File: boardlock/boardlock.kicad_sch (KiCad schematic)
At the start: 0 parts

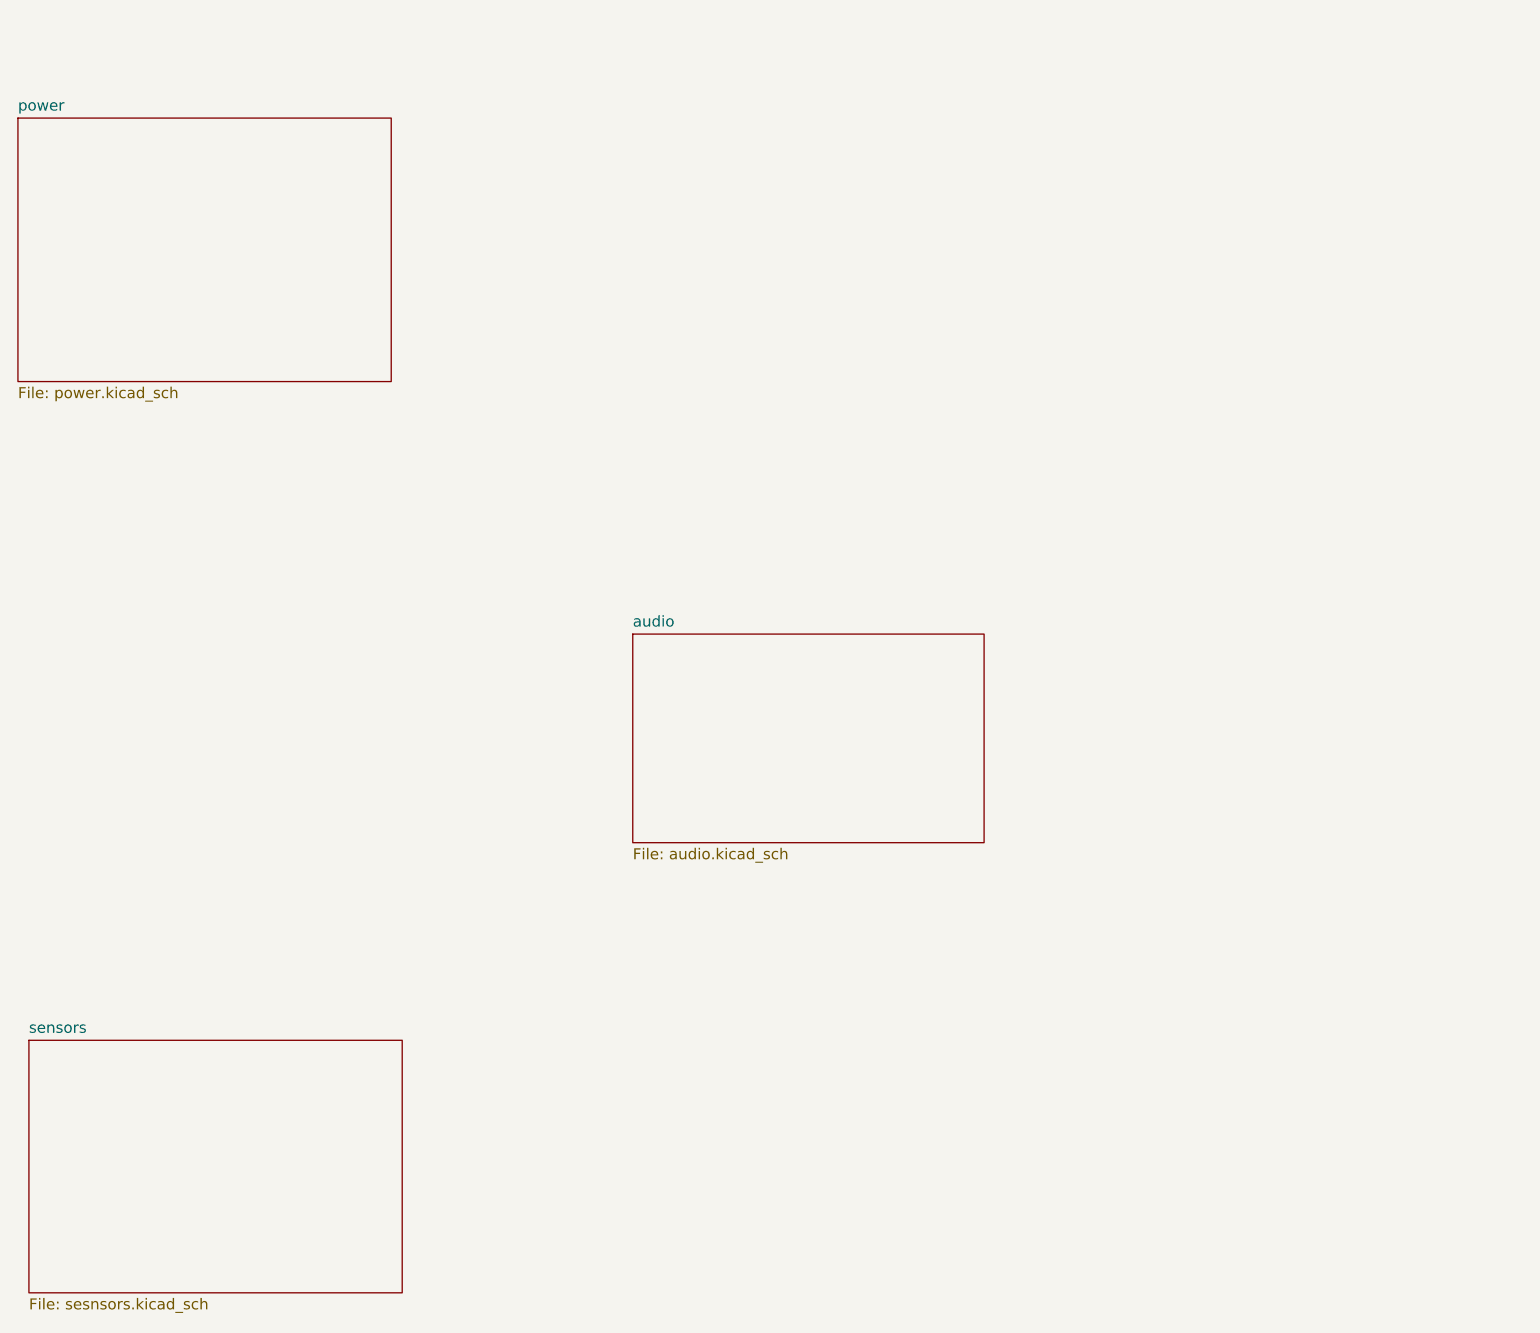
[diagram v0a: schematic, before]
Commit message: update
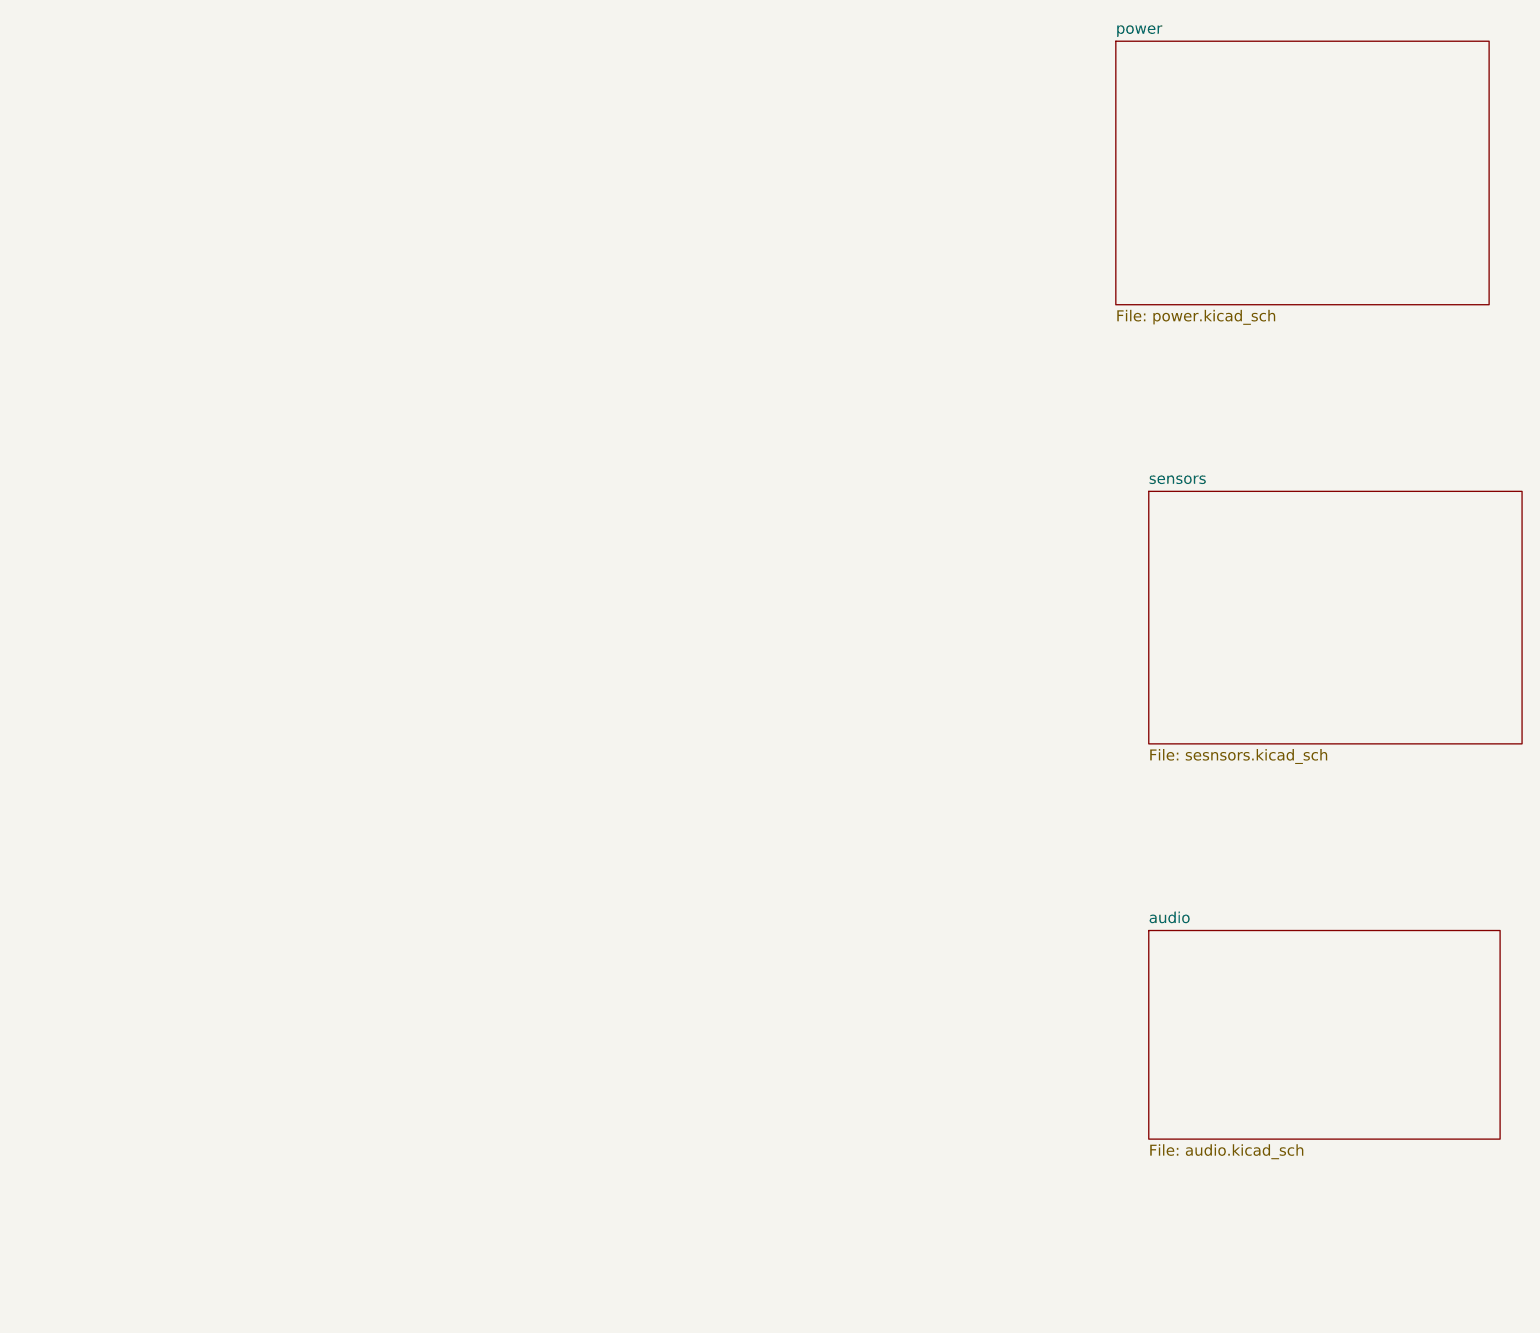
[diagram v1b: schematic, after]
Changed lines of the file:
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@@
 (kicad_sch (version 20230121) (generator eeschema)
   (paper "A4")
-  (sheet (at 62.23 140.97) (size 43.18 29.21) (fields_autoplaced)
+  (sheet (at 191.77 77.47) (size 43.18 29.21) (fields_autoplaced)
     (stroke (width 0.1524) (type solid))
     (fill (color 0 0 0 0.0000))
-    (property "Sheetname" "sensors" (at 62.23 140.2584 0)
+    (property "Sheetname" "sensors" (at 191.77 76.7584 0)
       (effects (font (size 1.27 1.27)) (justify left bottom))
     )
-    (property "Sheetfile" "sesnsors.kicad_sch" (at 62.23 170.7646 0)
+    (property "Sheetfile" "sesnsors.kicad_sch" (at 191.77 107.2646 0)
       (effects (font (size 1.27 1.27)) (justify left top))
     )
@@
     )
   )
-  (sheet (at 132.08 93.98) (size 40.64 24.13) (fields_autoplaced)
+  (sheet (at 191.77 128.27) (size 40.64 24.13) (fields_autoplaced)
     (stroke (width 0.1524) (type solid))
     (fill (color 0 0 0 0.0000))
-    (property "Sheetname" "audio" (at 132.08 93.2684 0)
+    (property "Sheetname" "audio" (at 191.77 127.5584 0)
       (effects (font (size 1.27 1.27)) (justify left bottom))
     )
-    (property "Sheetfile" "audio.kicad_sch" (at 132.08 118.6946 0)
+    (property "Sheetfile" "audio.kicad_sch" (at 191.77 152.9846 0)
       (effects (font (size 1.27 1.27)) (justify left top))
     )
@@
     )
   )
-  (sheet (at 60.96 34.29) (size 43.18 30.48) (fields_autoplaced)
+  (sheet (at 187.96 25.4) (size 43.18 30.48) (fields_autoplaced)
     (stroke (width 0.1524) (type solid))
     (fill (color 0 0 0 0.0000))
-    (property "Sheetname" "power" (at 60.96 33.5784 0)
+    (property "Sheetname" "power" (at 187.96 24.6884 0)
       (effects (font (size 1.27 1.27)) (justify left bottom))
     )
-    (property "Sheetfile" "power.kicad_sch" (at 60.96 65.3546 0)
+    (property "Sheetfile" "power.kicad_sch" (at 187.96 56.4646 0)
       (effects (font (size 1.27 1.27)) (justify left top))
     )
